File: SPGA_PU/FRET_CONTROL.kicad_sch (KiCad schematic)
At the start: 18 parts, among them U1 74HC595, U10 74HC595, U11 74HC595, U12 74HC595, U13 74HC595, U14 74HC595, U15 74HC595, U16 74HC595, U17 74HC595, U18 74HC595, U2 74HC595, U3 74HC595, U4 74HC595, U5 74HC595, U6 74HC595, U7 74HC595, U8 74HC595, U9 74HC595

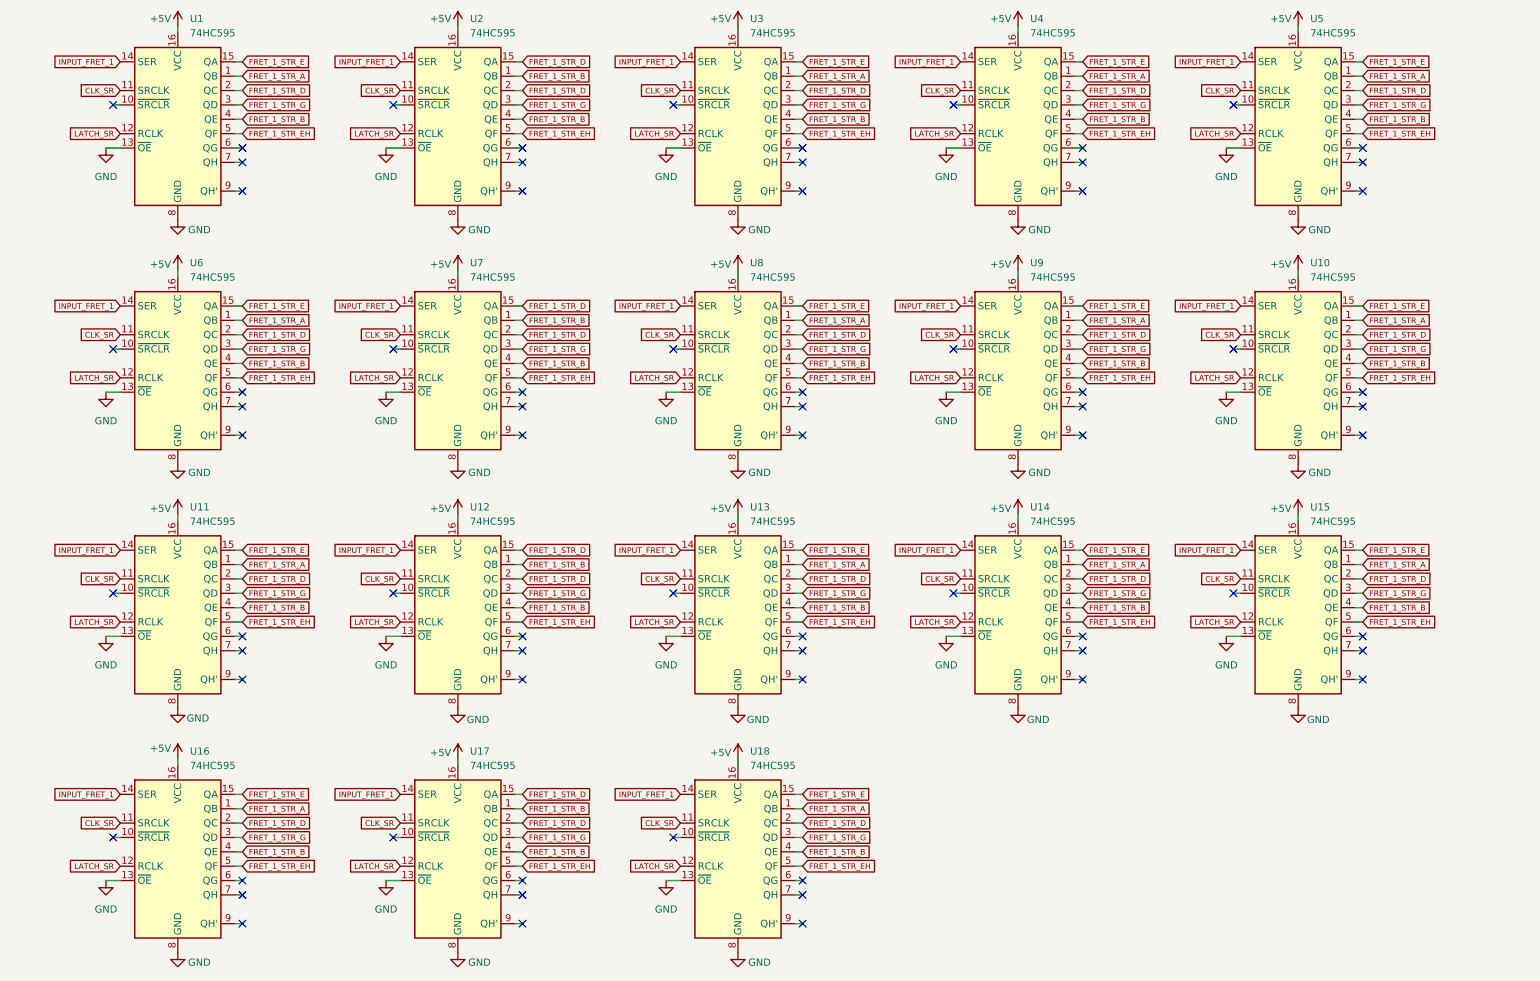
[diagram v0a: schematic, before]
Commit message: I dunno
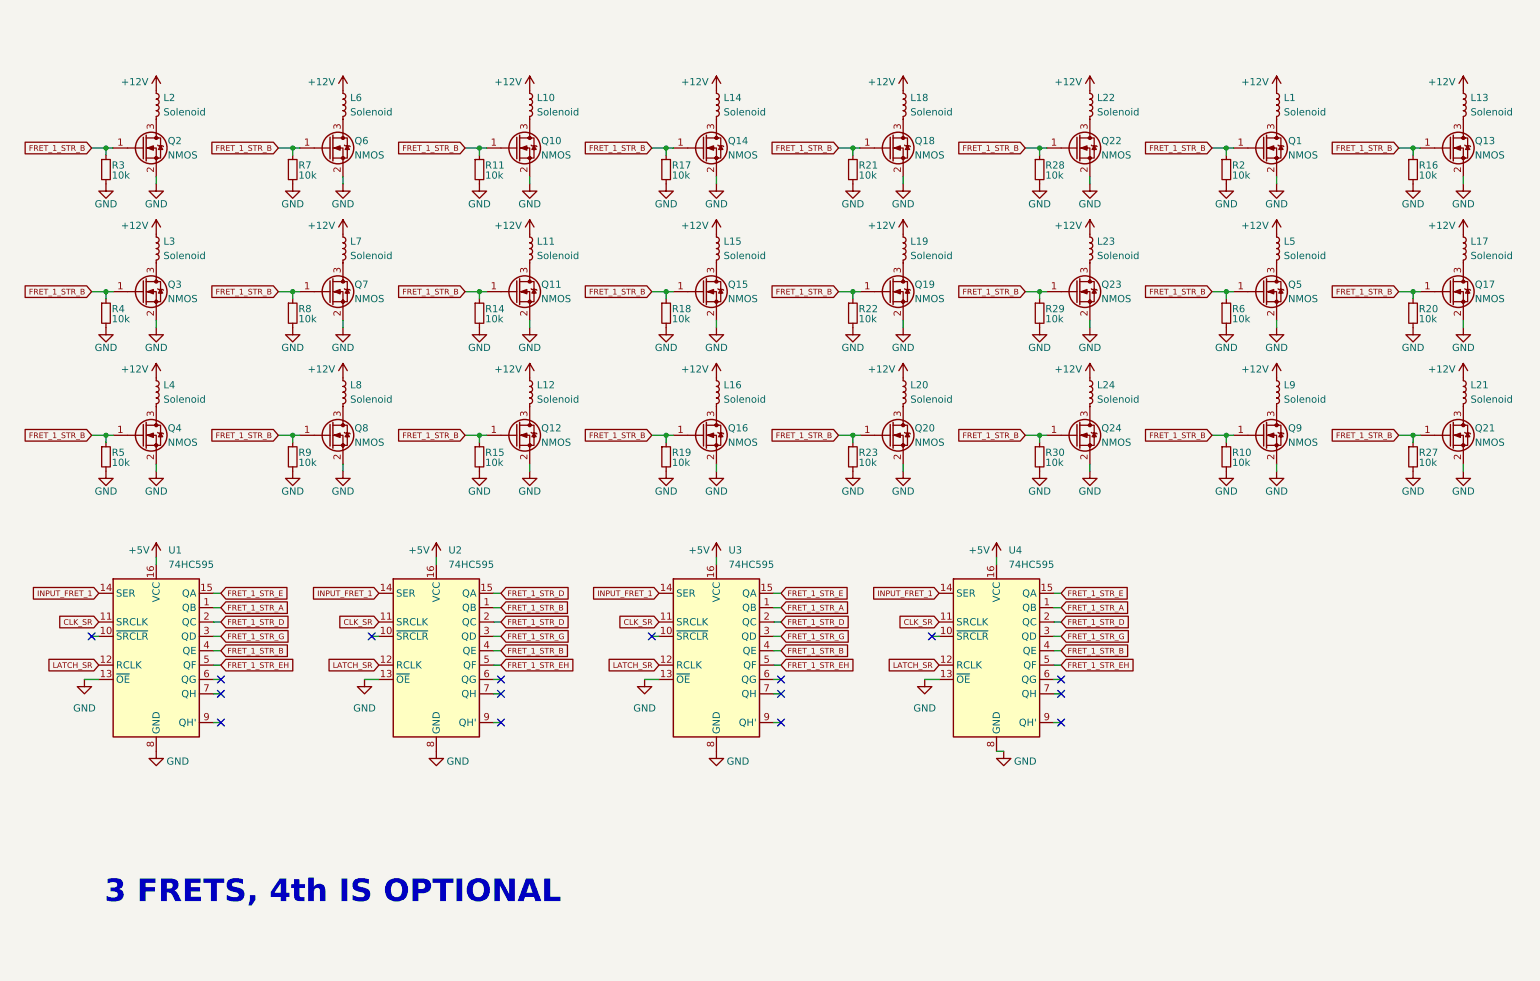
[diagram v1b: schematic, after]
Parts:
- removed U10, U11, U12, U13, U14, U15, U16, U17, U18, U5, U6, U7, U8, U9: 74HC595, symbol 74xx:74HC595
- added L1, L10, L11, L12, L13, L14, L15, L16, L17, L18, L19, L2, L20, L21, L22, L23, L24, L3, L4, L5, L6, L7, L8, L9: Solenoid, symbol Device:L_Small
- added Q1, Q10, Q11, Q12, Q13, Q14, Q15, Q16, Q17, Q18, Q19, Q2, Q20, Q21, Q22, Q23, Q24, Q3, Q4, Q5, Q6, Q7, Q8, Q9: NMOS, Package_TO_SOT_SMD:SOT-23-3, symbol Transistor_FET_Other:Q_NMOS_Depletion_GSD
- added R10, R11, R14, R15, R16, R17, R18, R19, R2, R20, R21, R22, R23, R27, R28, R29, R3, R30, R4, R5, R6, R7, R8, R9: 10k, symbol Device:R_Small
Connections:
- net FRET_1_STR_B: now also Q1.1 (G), Q10.1 (G), Q11.1 (G), Q12.1 (G), Q13.1 (G), Q14.1 (G), Q15.1 (G), Q16.1 (G), Q17.1 (G), Q18.1 (G), Q19.1 (G), Q2.1 (G), Q20.1 (G), Q21.1 (G), Q22.1 (G), Q23.1 (G), Q24.1 (G), Q3.1 (G), Q4.1 (G), Q5.1 (G), Q6.1 (G), Q7.1 (G), Q8.1 (G), Q9.1 (G), R10.1, R11.1, R14.1, R15.1, R16.1, R17.1, R18.1, R19.1, R2.1, R20.1, R21.1, R22.1, R23.1, R27.1, R28.1, R29.1, R3.1, R30.1, R4.1, R5.1, R6.1, R7.1, R8.1, R9.1
- net GND: now also Q1.2 (S), Q10.2 (S), Q11.2 (S), Q12.2 (S), Q13.2 (S), Q14.2 (S), Q15.2 (S), Q16.2 (S), Q17.2 (S), Q18.2 (S), Q19.2 (S), Q2.2 (S), Q20.2 (S), Q21.2 (S), Q22.2 (S), Q23.2 (S), Q24.2 (S), Q3.2 (S), Q4.2 (S), Q5.2 (S), Q6.2 (S), Q7.2 (S), Q8.2 (S), Q9.2 (S), R10.2, R11.2, R14.2, R15.2, R16.2, R17.2, R18.2, R19.2, R2.2, R20.2, R21.2, R22.2, R23.2, R27.2, R28.2, R29.2, R3.2, R30.2, R4.2, R5.2, R6.2, R7.2, R8.2, R9.2
- new net: L13.2, Q13.3 (D)
- new net: L2.2, Q2.3 (D)
- new net: L14.2, Q14.3 (D)
- new net: L7.2, Q7.3 (D)
- new net: L9.2, Q9.3 (D)
- new net: L4.2, Q4.3 (D)
- new net: L22.2, Q22.3 (D)
- new net: L6.2, Q6.3 (D)
- new net: L5.2, Q5.3 (D)
- new net: L11.2, Q11.3 (D)
- new net: L21.2, Q21.3 (D)
- new net: L1.2, Q1.3 (D)
- new net: L8.2, Q8.3 (D)
- new net: L3.2, Q3.3 (D)
- new net: L16.2, Q16.3 (D)
- new net: L15.2, Q15.3 (D)
- new net: L12.2, Q12.3 (D)
- new net: L18.2, Q18.3 (D)
- new net: L17.2, Q17.3 (D)
- new net: L23.2, Q23.3 (D)
- new net: L20.2, Q20.3 (D)
- new net: L10.2, Q10.3 (D)
- new net: L19.2, Q19.3 (D)
- new net: L24.2, Q24.3 (D)
- new net +12V: L1.1, L10.1, L11.1, L12.1, L13.1, L14.1, L15.1, L16.1, L17.1, L18.1, L19.1, L2.1, L20.1, L21.1, L22.1, L23.1, L24.1, L3.1, L4.1, L5.1, L6.1, L7.1, L8.1, L9.1
- no-connect marks 72 -> 16
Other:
- note added: "3 FRETS, 4th IS OPTIONAL"
- moved on the sheet: U1, U2, U3, U4
